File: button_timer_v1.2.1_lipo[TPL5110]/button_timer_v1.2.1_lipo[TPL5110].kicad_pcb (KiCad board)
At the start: 2 copper layers, 21 x 41.7 mm, 24 parts, among them J1 Conn_01x05_Female, Q1 TSM2301ACX, SW1 SW_Push, SW2 SW_Push, U1 TPL5110, U2 AP2112K-3.3, X1 ESP-12E

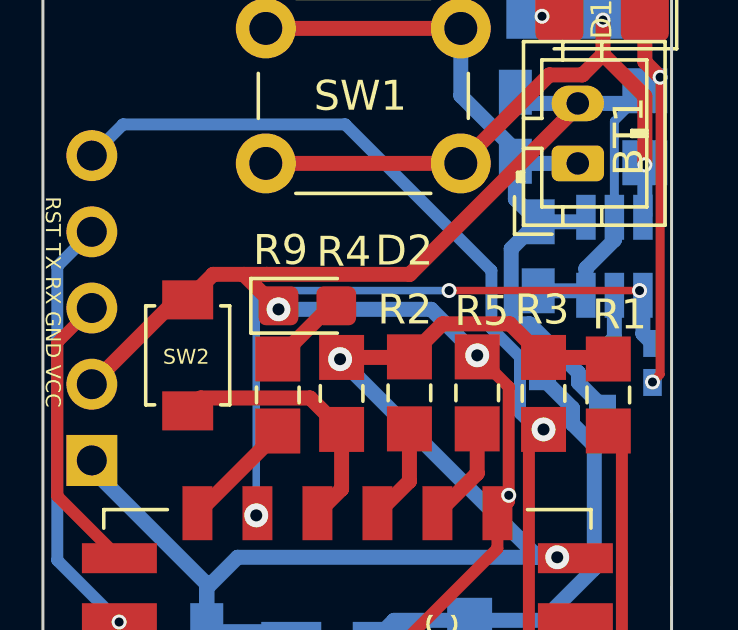
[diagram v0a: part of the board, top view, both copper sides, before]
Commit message: Silkscreen Update
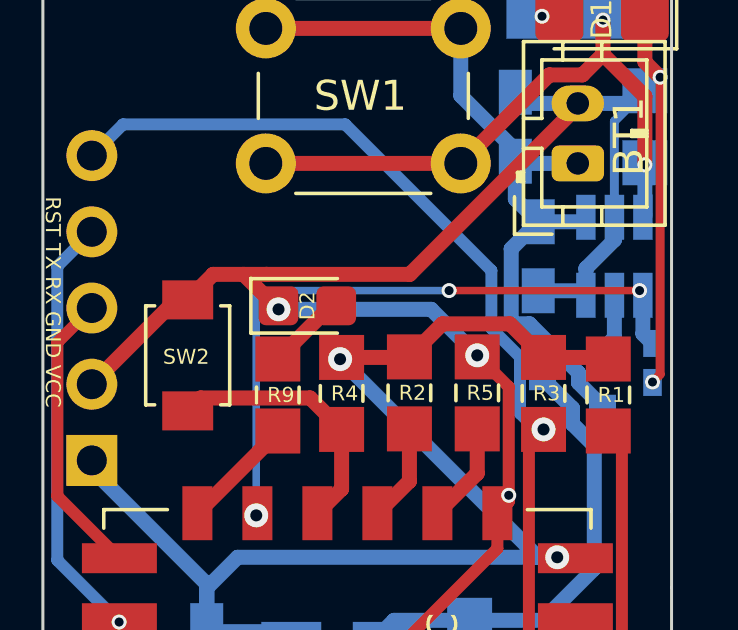
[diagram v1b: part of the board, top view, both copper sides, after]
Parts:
- D2: footprint LED_SMD:LED_0805_2012Metric_Castellated -> handsolder:LED_0805_2012Metric_Castellated_mod
- Q1: footprint Package_TO_SOT_SMD:SOT-23 -> handsolder:SOT-23_mod
